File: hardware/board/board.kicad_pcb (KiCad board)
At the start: 2 copper layers, 40.1 x 49.3 mm, 54 parts, among them J1 Eurorack Power, Q1 MMBT3904, U1 ATSAMD21G18A-AUT, U2 LM7805, U3 AP2112K-3.3, U4 LM4040DBZ-10, U5 TL072, U6 MCP6001-OT, U7 74AHCT1G125, U8 GD25Q64C

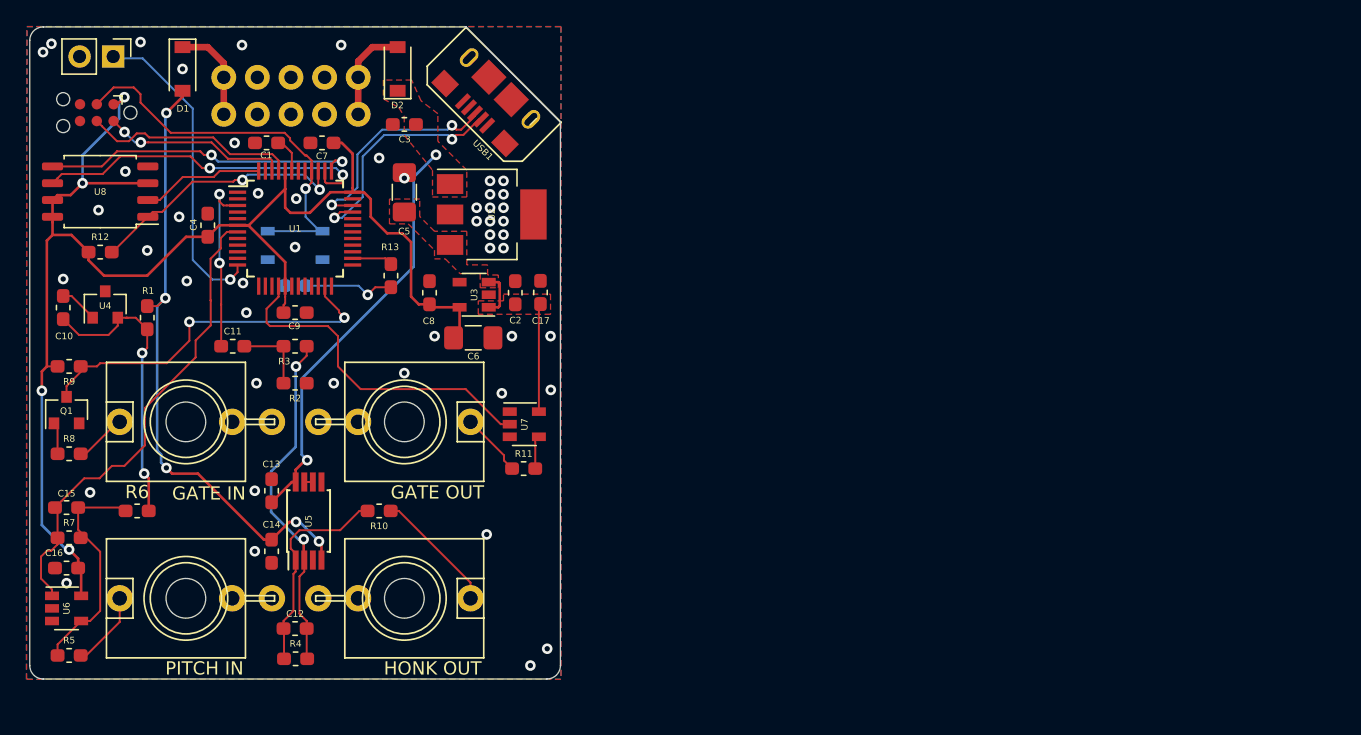
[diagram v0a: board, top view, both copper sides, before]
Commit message: done! apologies for no commits :-)
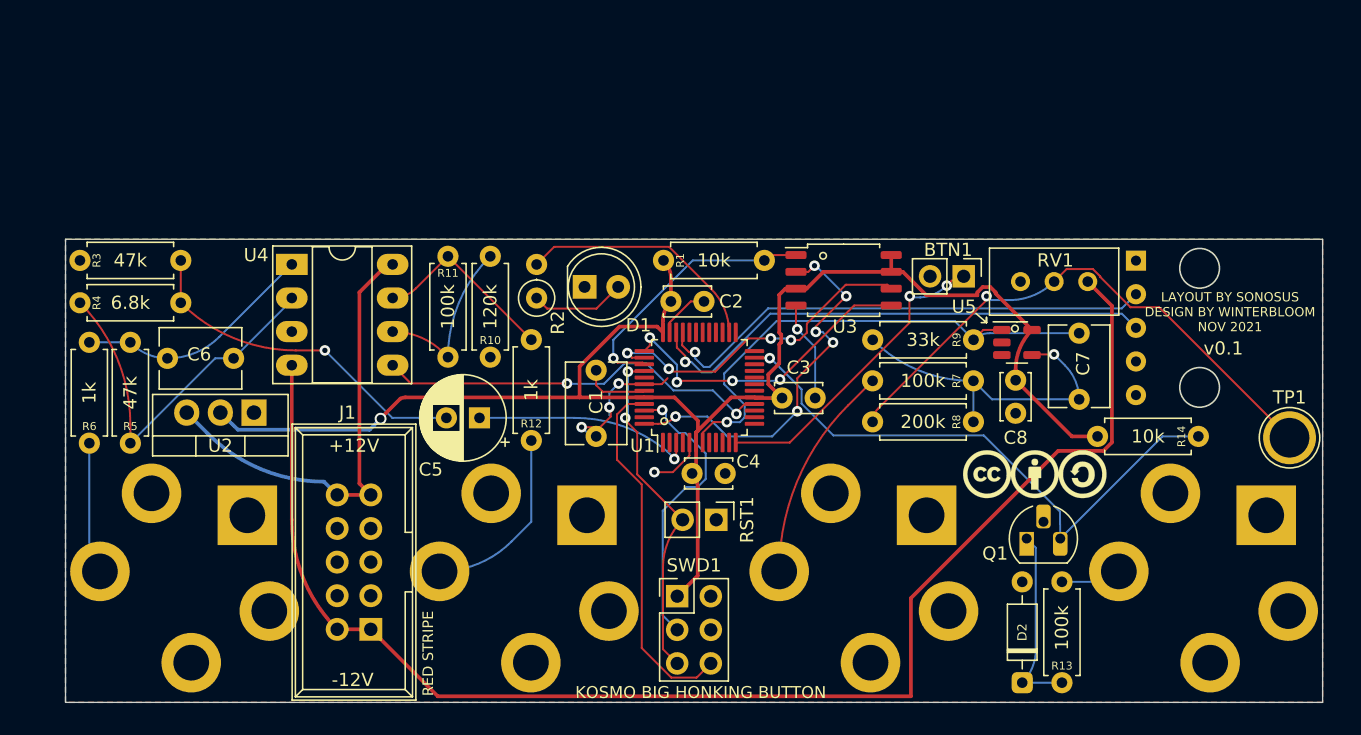
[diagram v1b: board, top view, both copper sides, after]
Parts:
- removed Button1: Big button, Connector_PinHeader_2.54mm:PinHeader_1x02_P2.54mm_Vertical
- removed C10, C13, C14, C16, C9: 0.1uF, Capacitor_SMD:C_0603_1608Metric_Pad1.05x0.95mm_HandSolder
- removed C11, C17: 1uF, Capacitor_SMD:C_0603_1608Metric_Pad1.05x0.95mm_HandSolder
- removed C12, C15: 18pF, Capacitor_SMD:C_0603_1608Metric_Pad1.05x0.95mm_HandSolder
- removed D3: LED, Diode_SMD:D_0603_1608Metric
- removed the G*** at (95.9, 121.1)
- removed REF**: OSHW-Logo2_7.3x6mm_SilkScreen, Symbol:OSHW-Logo2_7.3x6mm_SilkScreen
- removed RESET1: TACT_4.2MM, MF_Switches:MF_Switches-TACT4.2MM
- removed U6: MCP6001-OT, Package_TO_SOT_SMD:SOT-23-5
- removed U7: 74AHCT1G125, Package_TO_SOT_SMD:SOT-23-5
- removed U8: GD25Q64C, Package_SO:SOIC-8_5.23x5.23mm_P1.27mm
- added BTN1: Big button, Connector_PinHeader_2.54mm:PinHeader_1x02_P2.54mm_Vertical, F.Cu at (147.9, 117.8)
- added R14: 10k, Sonosus:Resistor, F.Cu at (165.6, 129.9)
- added RST1: TACT_4.2MM, Connector_PinHeader_2.54mm:PinHeader_1x02_P2.54mm_Vertical, F.Cu at (129.2, 136.2)
- added RV1: R_POT_TRIM, Potentiometer_THT:Potentiometer_Bourns_3296W_Vertical, F.Cu at (157.2, 118.2)
- added TP1: -10V test point, TestPoint:TestPoint_Plated_Hole_D3.0mm, F.Cu at (172.5, 130.0)
- C1: footprint Capacitor_SMD:C_0603_1608Metric_Pad1.05x0.95mm_HandSolder -> Sonosus:Capacitor_NonPolarized
- C2, C3, C8: value 1uF -> 0.1uF; footprint Capacitor_SMD:C_0603_1608Metric_Pad1.05x0.95mm_HandSolder -> Sonosus:Capacitor_NonPolarizedSmall
- C4: footprint Capacitor_SMD:C_0603_1608Metric_Pad1.05x0.95mm_HandSolder -> Sonosus:Capacitor_NonPolarizedSmall
- C5: value 10uF -> 1uF; footprint Capacitor_SMD:C_1206_3216Metric_Pad1.42x1.75mm_HandSolder -> Sonosus:Capacitor_Polarized
- C6: value 10uF -> 18pF; footprint Capacitor_SMD:C_1206_3216Metric_Pad1.42x1.75mm_HandSolder -> Sonosus:Capacitor_NonPolarized
- C7: value 0.1uF -> 18pF; footprint Capacitor_SMD:C_0603_1608Metric_Pad1.05x0.95mm_HandSolder -> Sonosus:Capacitor_NonPolarized
- CV_IN1, GATE_IN1, GATE_OUT1, HONK_OUT1: footprint board:WQP-PJ301M-12_JACK -> Sonosus:Jack_6.35mm_PJ_629HAN; moved to B.Cu
- D1: value D -> LED; footprint Diode_SMD:D_SOD-123 -> LED_THT:LED_D5.0mm
- D2: footprint Diode_SMD:D_SOD-123 -> Sonosus:Diode_DO-35
- G***: moved to F.Cu
- J1: footprint SF Connectors:2X5-SHROUDED_LOCK -> Sonosus:Power_Header; moved to F.Cu
- Q1: footprint Package_TO_SOT_SMD:SOT-23 -> Sonosus:Transistor_TO-92
- R1: value 2.2k -> 10k; footprint Resistor_SMD:R_0603_1608Metric_Pad1.05x0.95mm_HandSolder -> Sonosus:Resistor
- R10: value 1k -> 120k; footprint Resistor_SMD:R_0603_1608Metric_Pad1.05x0.95mm_HandSolder -> Sonosus:Resistor
- R11, R13: value 1k -> 100k; footprint Resistor_SMD:R_0603_1608Metric_Pad1.05x0.95mm_HandSolder -> Sonosus:Resistor
- R12: value 10k -> 1k; footprint Resistor_SMD:R_0603_1608Metric_Pad1.05x0.95mm_HandSolder -> Sonosus:Resistor
- R2: value 47k -> 1k; footprint Resistor_SMD:R_0603_1608Metric_Pad1.05x0.95mm_HandSolder -> Resistor_THT:R_Axial_DIN0207_L6.3mm_D2.5mm_P2.54mm_Vertical
- R3: value 6.8k -> 47k; footprint Resistor_SMD:R_0603_1608Metric_Pad1.05x0.95mm_HandSolder -> Sonosus:Resistor
- R4: value 47k -> 6.8k; footprint Resistor_SMD:R_0603_1608Metric_Pad1.05x0.95mm_HandSolder -> Sonosus:Resistor
- R5: value 100k -> 47k; footprint Resistor_SMD:R_0603_1608Metric_Pad1.05x0.95mm_HandSolder -> Sonosus:Resistor
- R6: value 200k -> 1k; footprint Resistor_SMD:R_0603_1608Metric_Pad1.05x0.95mm_HandSolder -> Sonosus:Resistor
- R7: value 33k -> 100k; footprint Resistor_SMD:R_0603_1608Metric_Pad1.05x0.95mm_HandSolder -> Sonosus:Resistor
- R8: value 100k -> 200k; footprint Resistor_SMD:R_0603_1608Metric_Pad1.05x0.95mm_HandSolder -> Sonosus:Resistor
- R9: value 10k -> 33k; footprint Resistor_SMD:R_0603_1608Metric_Pad1.05x0.95mm_HandSolder -> Sonosus:Resistor
- SWD1: footprint Connector:Tag-Connect_TC2030-IDC-NL_2x03_P1.27mm_Vertical -> Connector_PinHeader_2.54mm:PinHeader_2x03_P2.54mm_Vertical
- U2: value LM7805 -> LM1117-3.3; footprint Package_TO_SOT_SMD:SOT-223-3_TabPin2 -> Sonosus:Regulator_TO-220-3
- U3: value AP2112K-3.3 -> GD25Q64C; footprint Package_TO_SOT_SMD:SOT-23-5 -> Package_SO:SOIC-8_5.23x5.23mm_P1.27mm
- U4: value LM4040DBZ-10 -> TL072; footprint Package_TO_SOT_SMD:SOT-23 -> Sonosus:DIP-8_Socket
- U5: value TL072 -> MCP6001-OT; footprint Package_SO:TSSOP-8_4.4x3mm_P0.65mm -> Package_TO_SOT_SMD:SOT-23-5
- USB1: footprint MF_Connectors:MF_Connectors-MICROUSB-RIGHT -> Sonosus:Connector_USB_Micro_Tayda_A-5228; moved to B.Cu
- moved GATE_IN1 77.8 mm to (166.0, 140.6), turned to 0 degrees
- moved Q1 73.2 mm to (152.6, 137.6), turned to 0 degrees
- moved R7 69.4 mm to (148.6, 125.7), turned to 180 degrees
- moved R8 68.4 mm to (148.6, 128.8), turned to 180 degrees
- moved R9 68.4 mm to (148.6, 122.6)
- moved D2 66.2 mm to (152.3, 148.5)
- moved USB1 64.0 mm to (175.0, 115.0), turned to 180 degrees
- moved R13 59.3 mm to (155.3, 148.5)
- moved C7 59.0 mm to (156.6, 122.1), turned to -90 degrees
- moved SWD1 57.1 mm to (126.2, 142.0), turned to 0 degrees
- moved G*** 56.0 mm to (153.2, 132.8), turned to 0 degrees
- moved U5 55.2 mm to (151.9, 122.8), turned to 0 degrees
- moved CV_IN1 51.3 mm to (140.3, 140.6), turned to 0 degrees
- moved C8 44.8 mm to (151.8, 125.7), turned to -90 degrees
- moved C4 41.1 mm to (127.3, 132.7), turned to 0 degrees
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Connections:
- C2 pad 1: +5V -> +3V3
- C3 pad 1: +12V -> +3V3
- C5 pad 1: +5V -> A0
- C5 pad 2: GND -> Net-(C5-Pad2)
- C6 pad 1: +3V3 -> Net-(C6-Pad1)
- C6 pad 2: GND -> Net-(C6-Pad2)
- C7 pad 1: +3V3 -> A1
- C7 pad 2: GND -> Net-(C7-Pad2)
- D1 pad 1: Net-(D1-Pad1) -> GND
- D1 pad 2: -12V -> Net-(D1-Pad2)
- D2 pad 1: +12V -> Net-(D2-Pad1)
- D2 pad 2: Net-(D2-Pad2) -> GND
- J1 pad 1: Net-(D1-Pad1) -> -12V
- J1 pad 10: Net-(D2-Pad2) -> +12V
- J1 pad 2: Net-(D1-Pad1) -> -12V
- J1 pad 9: Net-(D2-Pad2) -> +12V
- Q1 pad 1: Net-(Q1-Pad1) -> Net-(D2-Pad1)
- R1 pad 1: VREF_-10 -> +3V3
- R1 pad 2: -12V -> FLASH_CS
- R10 pad 1: AUDIO_OUT -> GND
- R10 pad 2: Net-(C12-Pad1) -> Net-(R10-Pad2)
- R11 pad 1: GATE_OUT -> Net-(R11-Pad1)
- R11 pad 2: Net-(R11-Pad2) -> Net-(R10-Pad2)
- R12 pad 1: +3V3 -> GATE_OUT
- R12 pad 2: FLASH_CS -> Net-(R11-Pad1)
- R13 pad 1: Net-(D3-Pad2) -> Net-(D2-Pad1)
- R13 pad 2: D13 -> GATE_IN
- R2 pad 1: GND -> Net-(D1-Pad2)
- R2 pad 2: Net-(C11-Pad2) -> D13
- R3 pad 1: Net-(C12-Pad2) -> GND
- R3 pad 2: Net-(C11-Pad2) -> Net-(C5-Pad2)
- R4 pad 1: Net-(C12-Pad2) -> Net-(C6-Pad2)
- R4 pad 2: Net-(C12-Pad1) -> Net-(C5-Pad2)
- R5 pad 1: Net-(C15-Pad2) -> Net-(C6-Pad2)
- R5 pad 2: CV_IN -> Net-(C6-Pad1)
- R6 pad 1: Net-(C15-Pad2) -> AUDIO_OUT
- R6 pad 2: VREF_-10 -> Net-(C6-Pad1)
- R7 pad 1: A1 -> Net-(C7-Pad2)
- R7 pad 2: Net-(C15-Pad2) -> CV_IN
- R8 pad 1: Net-(Q1-Pad1) -> Net-(C7-Pad2)
- R8 pad 2: GATE_IN -> VREF_-10
- R9 pad 1: D2 -> A1
- R9 pad 2: +3V3 -> Net-(C7-Pad2)
- SWD1 pad 2: SWDIO -> unconnected-(SWD1-Pad2)
- SWD1 pad 3: RESET -> SWDIO
- SWD1 pad 4: SWCLK -> GND
- SWD1 pad 5: GND -> RESET
- SWD1 pad 6: Net-(SWD1-Pad6) -> SWCLK
- U1 pad 1: Net-(U1-Pad1) -> unconnected-(U1-Pad1)
- U1 pad 2: Net-(U1-Pad2) -> unconnected-(U1-Pad2)
- U1 pad 20: Net-(U1-Pad20) -> unconnected-(U1-Pad20)
- U1 pad 21: Net-(U1-Pad21) -> unconnected-(U1-Pad21)
- U1 pad 22: Net-(U1-Pad22) -> unconnected-(U1-Pad22)
- U1 pad 31: Net-(U1-Pad31) -> unconnected-(U1-Pad31)
- U1 pad 32: Net-(U1-Pad32) -> unconnected-(U1-Pad32)
- U1 pad 4: Net-(U1-Pad4) -> unconnected-(U1-Pad4)
- U1 pad 41: Net-(U1-Pad41) -> unconnected-(U1-Pad41)
- U2 pad 1: +12V -> GND
- U2 pad 2: GND -> +3V3
- U2 pad 3: +5V -> +12V
- U3 pad 1: +5V -> FLASH_CS
- U3 pad 2: GND -> FLASH_MISO
- U3 pad 3: +5V -> +3V3
- U3 pad 4: Net-(U3-Pad4) -> GND
- U3 pad 5: +3V3 -> FLASH_MOSI
- U4 pad 1: GND -> Net-(C6-Pad1)
- U4 pad 2: VREF_-10 -> Net-(C6-Pad2)
- U4 pad 3: (no net) -> GND
- U5 pad 1: Net-(C12-Pad1) -> A1
- U5 pad 2: Net-(C12-Pad2) -> GND
- U5 pad 4: -12V -> Net-(C7-Pad2)
- U5 pad 5: GND -> +3V3
- USB1 pad 1: Net-(USB1-Pad1) -> unconnected-(USB1-Pad1)
- USB1 pad 4: Net-(USB1-Pad4) -> unconnected-(USB1-Pad4)
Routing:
- net -12V: track 47.7 -> 106.7 mm, vias 5 -> 0
- net Net-(C6-Pad2): track 0.00 -> 28.4 mm
- net Net-(C12-Pad2): track 26.4 -> 0.00 mm, vias 2 -> 0
- net Net-(C5-Pad2): track 0.00 -> 26.3 mm, vias 0 -> 1
- net Net-(C7-Pad2): track 0.00 -> 25.7 mm, vias 0 -> 1
- net GND: track 3.11 -> 27.0 mm, vias 49 -> 5
- net D+: track 17.1 -> 39.2 mm, vias 2 -> 1
- net D-: track 17.8 -> 38.5 mm, vias 2 -> 1
- net FLASH_MISO: track 9.29 -> 29.7 mm, vias 0 -> 6
- net VREF_-10: track 22.3 -> 42.1 mm, vias 2 -> 1
- net Net-(C6-Pad1): track 0.00 -> 18.3 mm
- net Net-(C15-Pad2): track 17.4 -> 0.00 mm
- net D2: track 27.8 -> 44.2 mm, vias 2 -> 1
- net Net-(C12-Pad1): track 16.3 -> 0.00 mm
- net D13: track 3.07 -> 18.7 mm
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- removed copper zone on F.Cu, net +12V
- removed copper zone on F.Cu, net +5V
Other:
- board size 40.1 x 49.3 mm -> 95 x 35 mm
- net class Default removed
- rule pad_to_mask_clearance: 0.051 -> 0
- board text added: "KOSMO BIG HONKING BUTTON"
- board text added: "LAYOUT BY SONOSUS DESIGN BY WINTERBLOOM NOV 2021"
- board text added: "v0.1"
- board text removed: "Big Honking Button"
- board text removed: "GATE IN"
- board text removed: "GATE OUT"
- board text removed: "HONK OUT"
- board text removed: "PITCH IN"
- board text removed: "RED STRIPE"
- board text removed: "TRANS RIGHTS"
- board text removed: "v5 10/7/2020 CC BY-SA 4.0 wntr.dev/honk"
